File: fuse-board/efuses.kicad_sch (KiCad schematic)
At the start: 72 parts, among them U10 TPS259830ONRGER, U11 TPS259830ONRGER, U12 TPS259830ONRGER, U4 TPS259830ONRGER, U5 TPS259830ONRGER, U6 TPS259830ONRGER, U7 TPS259830ONRGER, U8 TPS259830ONRGER, U9 TPS259830ONRGER

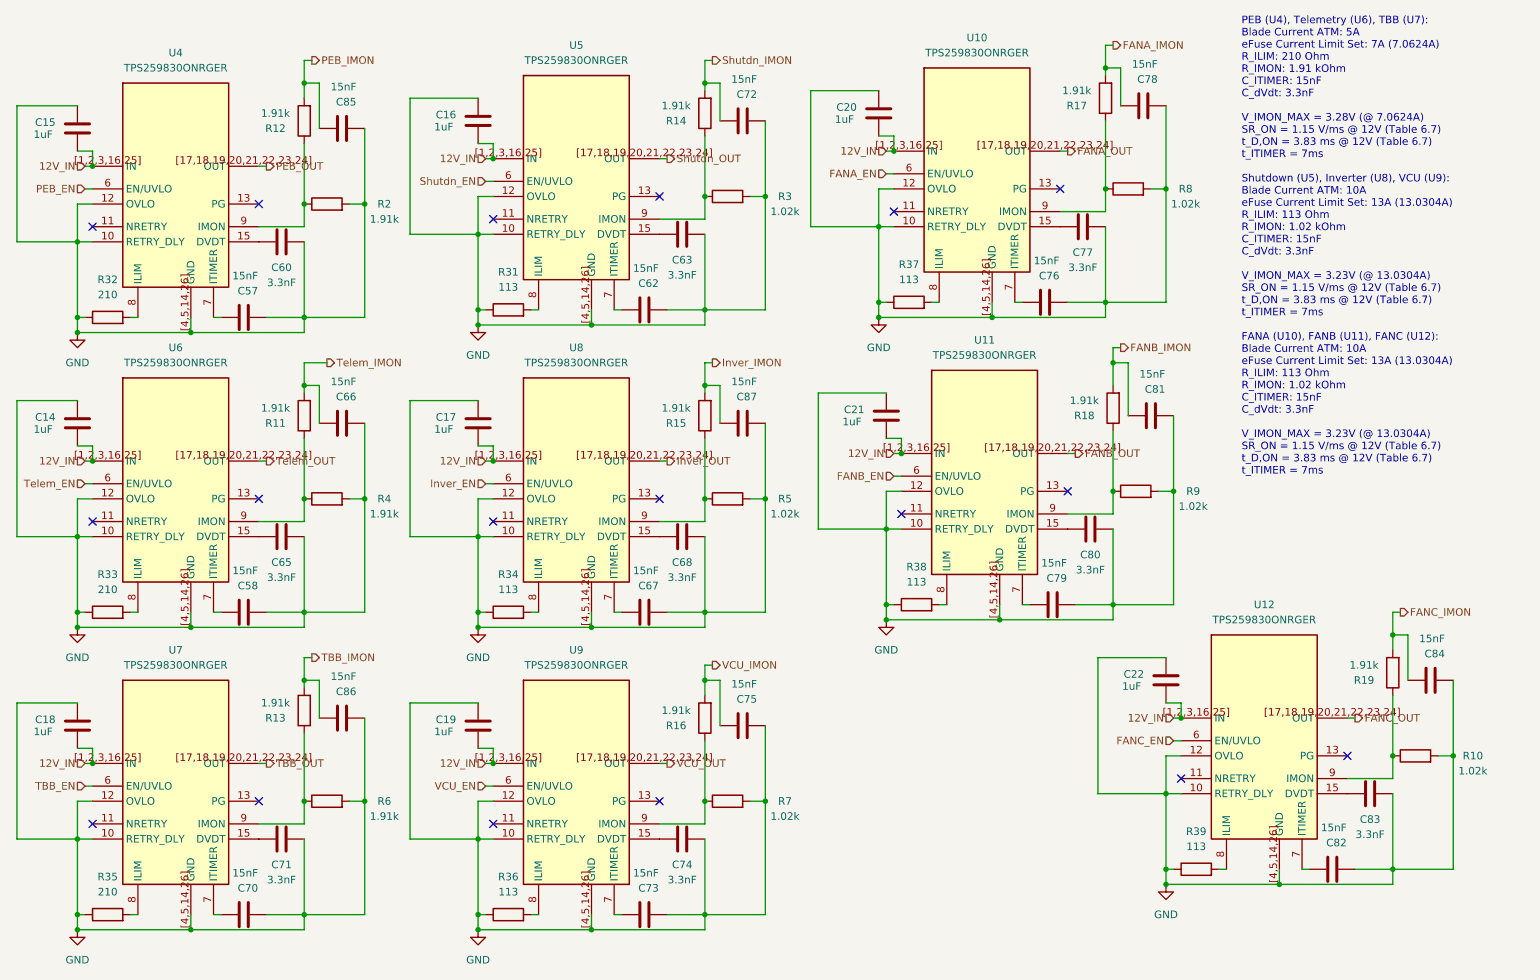
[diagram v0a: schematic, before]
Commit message: update to have >10kohm series r
reccomended by TI in datasheet
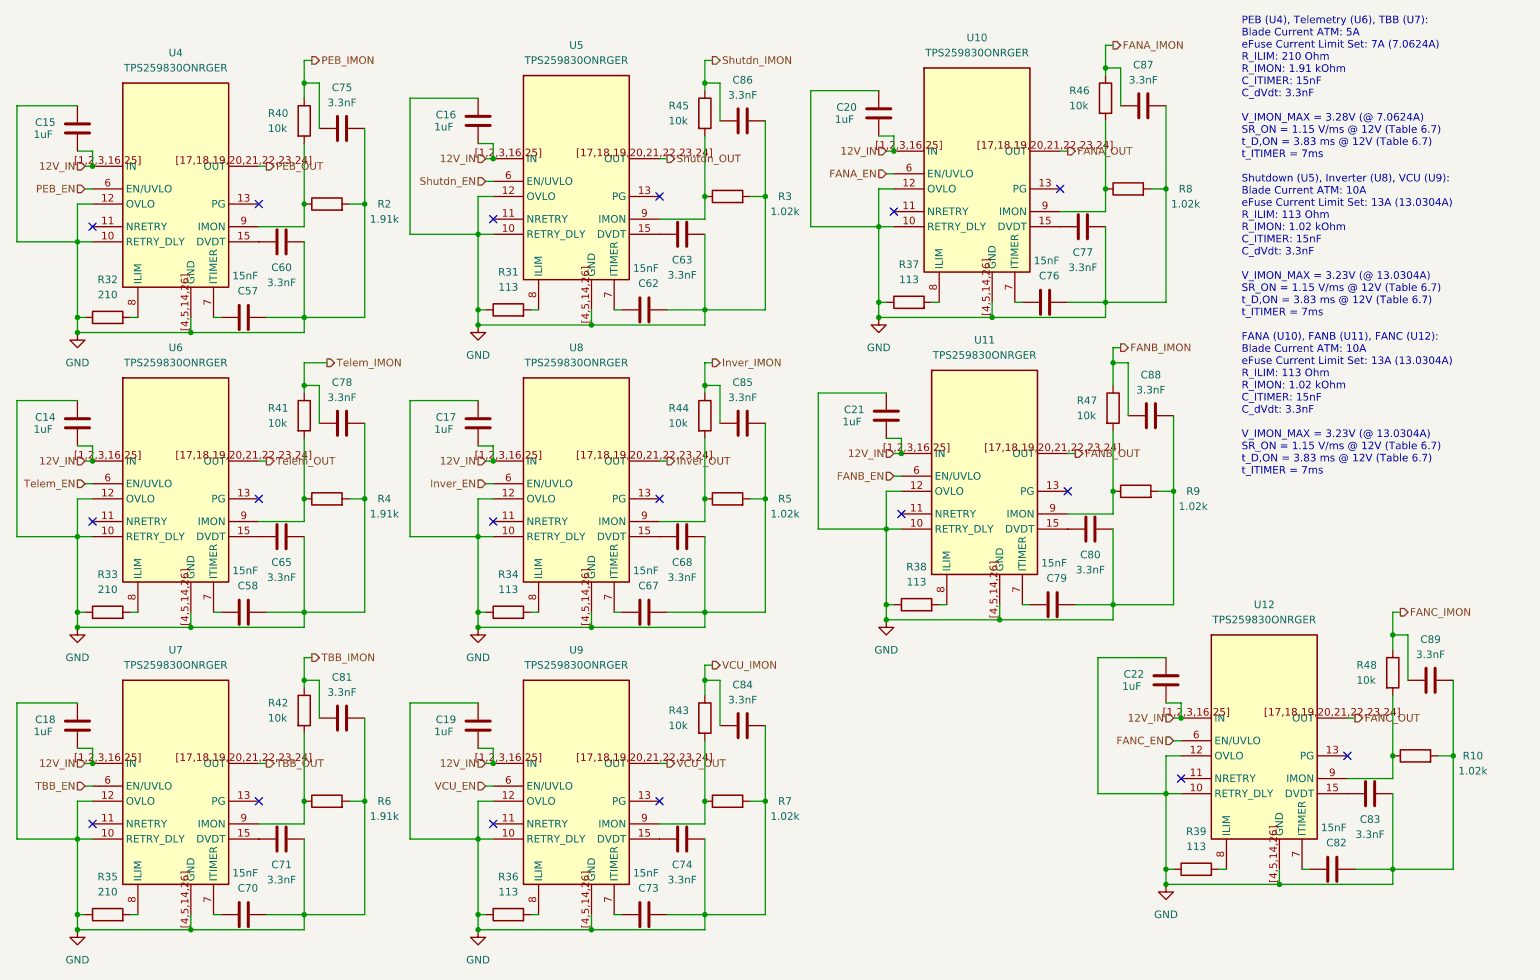
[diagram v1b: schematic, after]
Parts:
- removed C66, C72: 15nF, Capacitor_SMD:C_0603_1608Metric_Pad1.08x0.95mm_HandSolder, symbol Device:C
- removed R11, R12, R13, R14, R15, R16, R17, R18, R19: 1.91k, Resistor_SMD:R_0603_1608Metric_Pad0.98x0.95mm_HandSolder, symbol Device:R
- added C88, C89: 3.3nF, Capacitor_SMD:C_0603_1608Metric_Pad1.08x0.95mm_HandSolder, symbol Device:C
- added R40, R41, R42, R43, R44, R45, R46, R47, R48: 10k, Resistor_SMD:R_0603_1608Metric_Pad0.98x0.95mm_HandSolder, symbol Device:R
- C75, C78, C81, C84, C85, C86, C87: value 15nF -> 3.3nF; Digikey Part Number 311-1430-1-ND -> 311-1082-1-ND; Digikey URL https://www.digikey.com/en/products/detail/yageo/CC0603KRX7R9BB153/2833595?s=N4IgjCBcoEwAwBYCcVQAcAuUQFUB2AlhgPIBmAsgKYCGAzgK4BOlIANCPdmgGJsgC2BPNjABWOBL79qADxHjJAX0XsYUANogAwlrgA2OAGYA0gCUAGgHZTSAEK2QAXUVA -> https://www.digikey.com/en/products/detail/yageo/CC0603KRX7R9BB332/302816?s=N4IgjCBcoEwAwBYCcVQAcAuUQFUB2AlhgPIBmAsgKYCGAzgK4BOlIANCPdmgGJsgC2BPNgDMIuHD79qAD1HjJAX0XsYUANogAwlrgA2OCIDSAJQAaAdhNIAQjZABdRUA; Manufacturer Part Number CC0603KRX7R9BB153 -> CC0603KRX7R9BB332
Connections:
- net FANA_IMON: now also C87.1, R46.1; no longer C78.1
- net FANB_IMON: now also C88.1, R47.1; no longer C81.1
- net FANC_IMON: now also C89.1, R48.1; no longer C84.1
- net GND: now also C88.2, C89.2
- net Inver_IMON: now also C85.1, R44.1; no longer C87.1
- net PEB_IMON: now also C75.1, R40.1; no longer C85.1
- net Shutdn_IMON: now also C86.1, R45.1
- net TBB_IMON: now also C81.1, R42.1; no longer C86.1
- net Telem_IMON: now also C78.1, R41.1
- net VCU_IMON: now also C84.1, R43.1; no longer C75.1
- net at R5.1, U8.9 (IMON): now also R44.2
- net at R2.1, U4.9 (IMON): now also R40.2
- net at R4.1, U6.9 (IMON): now also R41.2
- net at R3.1, U5.9 (IMON): now also R45.2
- net at R7.1, U9.9 (IMON): now also R43.2
- net at R6.1, U7.9 (IMON): now also R42.2
- net at R9.1, U11.9 (IMON): now also R47.2
- net at R8.1, U10.9 (IMON): now also R46.2
- net at R10.1, U12.9 (IMON): now also R48.2
